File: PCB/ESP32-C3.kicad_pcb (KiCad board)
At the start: 2 copper layers, 31 x 30 mm, 45 parts, among them J1 HCZZ0039-3, J2 DPS_PPS_Right_Angle, SW2 TS4535TP 250gf 009, U1 USB-C-16P-SMD, U2 BQ24072RGT, U3 ESP32-C3, Y1 40MHz_S3240000151040

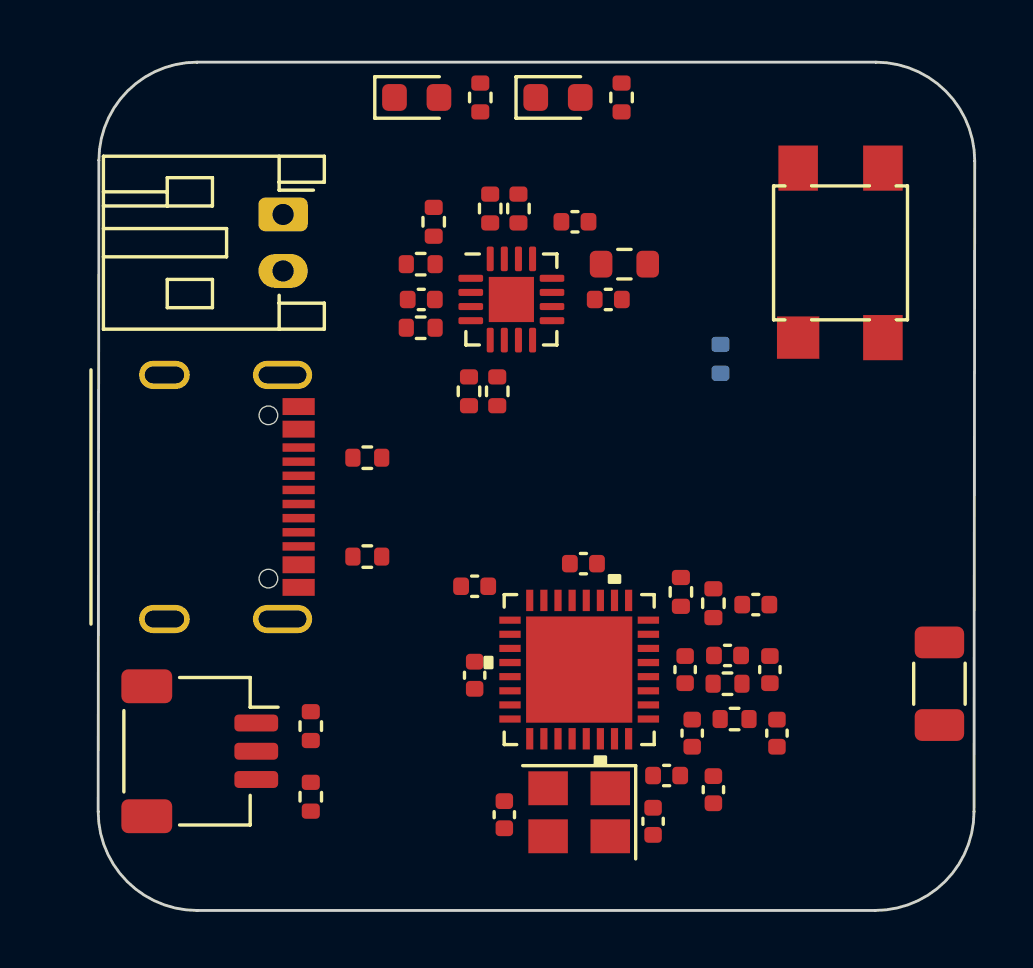
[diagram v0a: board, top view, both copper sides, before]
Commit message: Layout weiter gemacht.
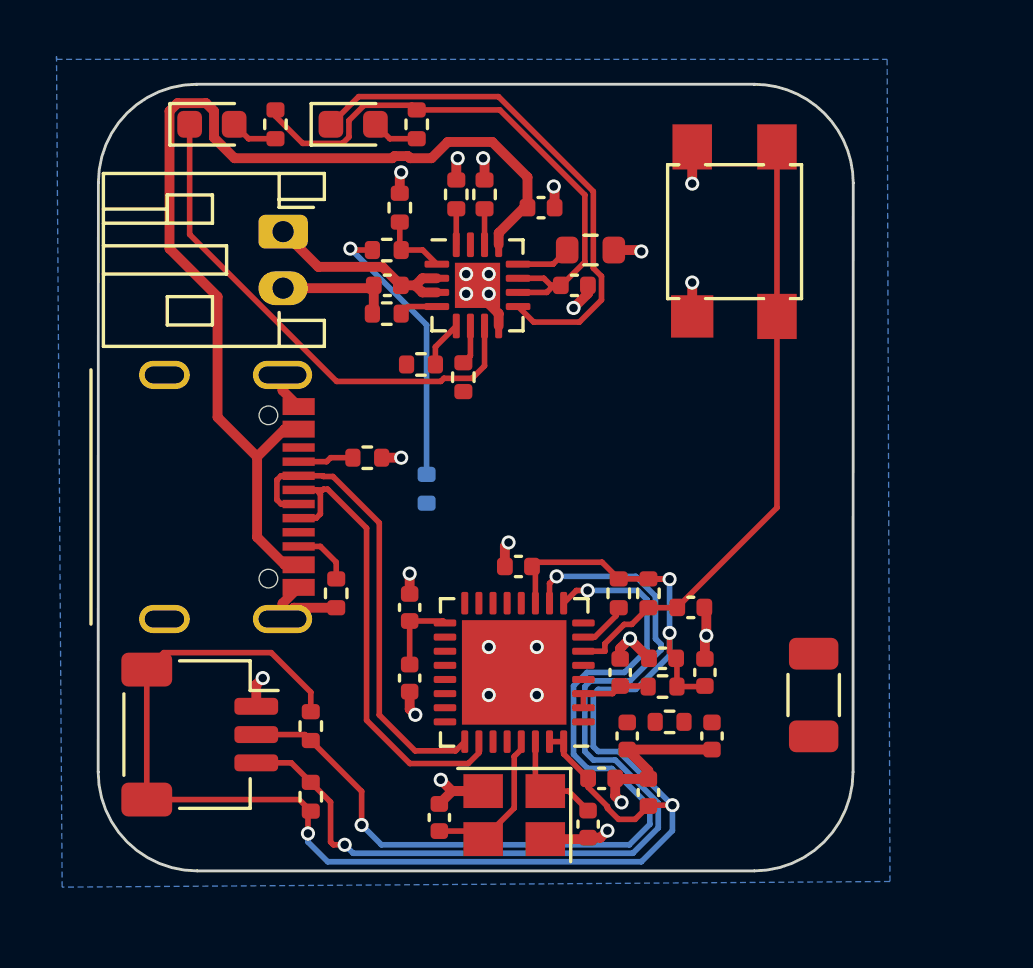
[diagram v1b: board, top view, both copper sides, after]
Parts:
- U3: footprint ESP32-C3:ESP32-C3 -> Package_DFN_QFN:QFN-32-1EP_5x5mm_P0.5mm_EP3.7x3.7mm
- moved R13 11.4 mm to (140.6, 82.6), turned to -90 degrees
- moved D4 7.31 mm to (133.0, 69.7)
- moved D5 7.31 mm to (138.0, 69.7)
- moved R10 7.31 mm to (135.2, 69.7)
- moved R9 7.31 mm to (140.2, 69.7)
- moved AE1 4.47 mm to (154.3, 89.9)
- moved SW2 3.82 mm to (151.5, 73.5)
- moved C14 2.42 mm to (140.0, 86.8), turned to 90 degrees
- moved R1 2.33 mm to (148.4, 86.3)
- moved Y1 2.30 mm to (143.7, 94.2)
- moved C1 2.30 mm to (149.9, 86.8)
- moved C11 2.30 mm to (140.0, 89.3)
- moved C12 2.30 mm to (146.8, 92.8)
- moved C15 2.30 mm to (148.4, 93.3)
- moved C16 2.30 mm to (146.3, 94.5)
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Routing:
- net +3.3V: track 0.00 -> 84.9 mm, vias 0 -> 4
- net GND: track 0.00 -> 38.2 mm, vias 0 -> 26
- net VCC: track 0.00 -> 38.0 mm
- net MCU_SDA: track 0.00 -> 33.4 mm, vias 0 -> 2
- net MCU_SCL: track 0.00 -> 31.2 mm, vias 0 -> 2
- net EXTI: track 0.00 -> 21.9 mm
- net NCHG: track 0.00 -> 18.5 mm
- net NPGOOD: track 0.00 -> 18.1 mm
- net USB_D+: track 0.00 -> 17.3 mm
- net USB_D-: track 0.00 -> 16.4 mm
- net Net-(R12-Pad2): track 0.00 -> 9.91 mm, vias 0 -> 1
- net +BATT: track 0.00 -> 7.20 mm
- net Net-(U3-XTAL_N): track 0.00 -> 5.68 mm
- net Net-(U3-XTAL_P): track 0.00 -> 3.70 mm
- net Net-(C7-Pad2): track 0.00 -> 2.91 mm
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- added copper zone on B.Cu, net GND
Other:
- board size 31 x 30 mm -> 26.7 x 27.8 mm
